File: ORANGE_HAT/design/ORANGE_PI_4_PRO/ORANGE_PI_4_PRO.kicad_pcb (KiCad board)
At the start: 2 copper layers, 58 x 26 mm, 6 parts, among them P1 Conn_02x20_Odd_Even, P2 Conn_02x20_Odd_Even

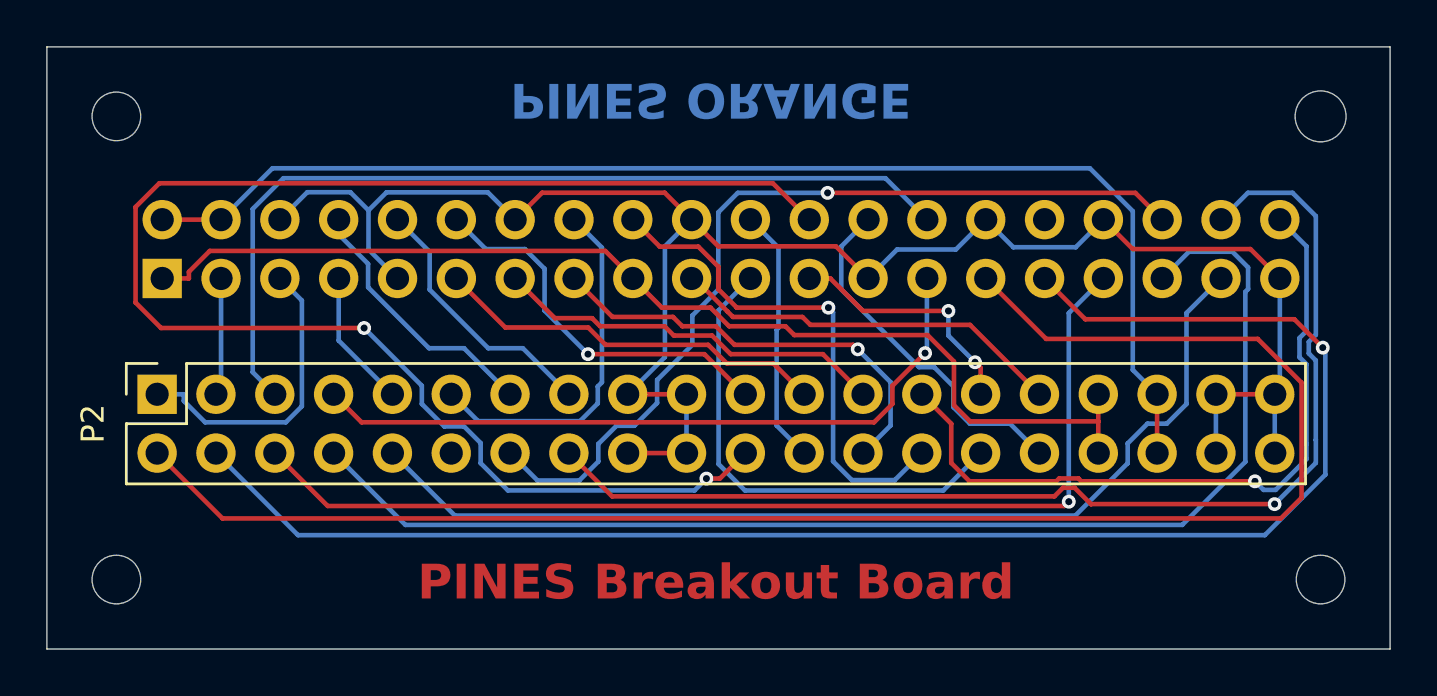
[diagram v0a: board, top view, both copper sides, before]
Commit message: feat: Git ignore
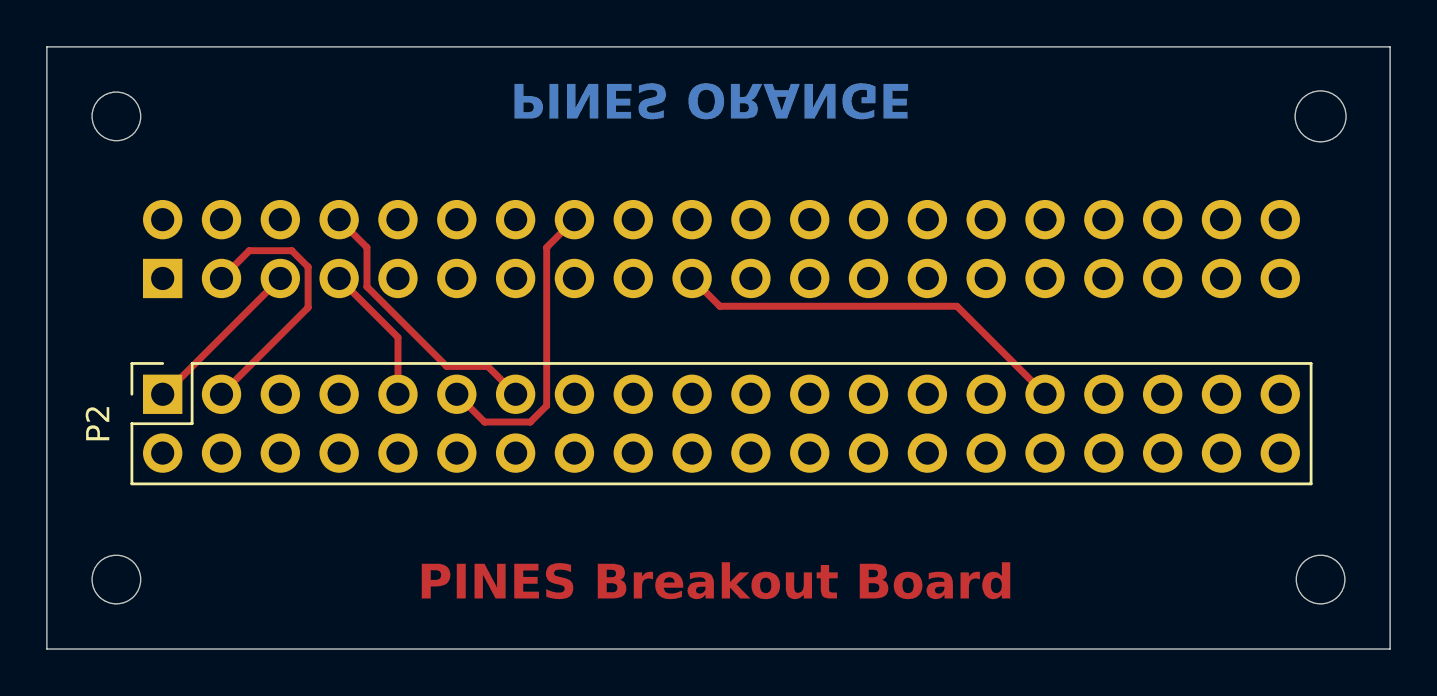
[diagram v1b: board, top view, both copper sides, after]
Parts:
- moved P2 0.24 mm to (209.0, 106.0)
- renumbered REF** to H1, REF** to H2, REF** to H3, REF** to H4
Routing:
- net GND: track 82.4 -> 0.00 mm
- net /PD0: track 71.4 -> 0.00 mm
- net /PD1: track 69.2 -> 0.00 mm, vias 1 -> 0
- net /PE12: track 65.6 -> 0.00 mm, vias 2 -> 0
- net /PD3: track 54.7 -> 0.00 mm
- net +5V: track 54.5 -> 0.00 mm
- net /PD7: track 50.1 -> 0.00 mm, vias 1 -> 0
- net +3.3V: track 47.8 -> 0.00 mm
- net /PD2: track 45.6 -> 0.00 mm, vias 1 -> 0
- net /PD4: track 43.9 -> 0.00 mm
- net /PB4: track 38.8 -> 0.00 mm
- net /PD6: track 38.0 -> 0.00 mm, vias 1 -> 0
- net /PL13: track 31.0 -> 0.00 mm, vias 1 -> 0
- net /PB5: track 31.0 -> 0.00 mm, vias 1 -> 0
- net /PK25: track 22.0 -> 0.00 mm, vias 1 -> 0
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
